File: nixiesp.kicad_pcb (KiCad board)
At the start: 2 copper layers, 152.4 x 53.3 mm, 51 parts, among them J1 Power 9-15V, J2 ESP8266, J3 Nixie PSU low, J4 CONN_01X02, Q1 BS107, Q2 BS107, Q3 BS107, Q4 BS107, U1 74HC595, U10 LM1117-3.3, U11 LM1117-3.3, U2 K155ID1, U3 K155ID1, U4 K155ID1, U5 74HC595, U6 K155ID1, U7 K155ID1, U8 74HC595, U9 K155ID1

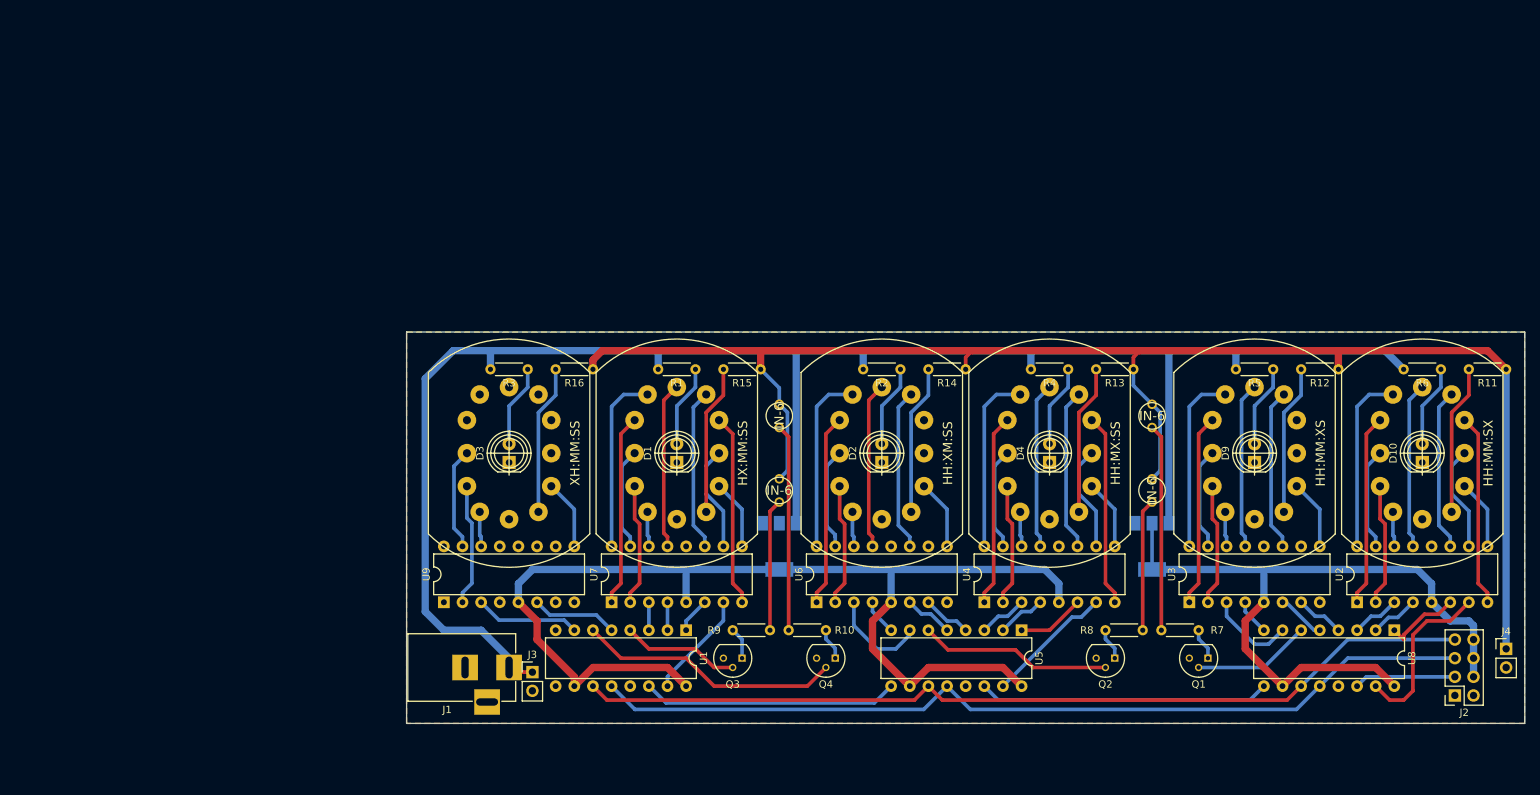
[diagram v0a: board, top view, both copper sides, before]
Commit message: Hopefully final changes
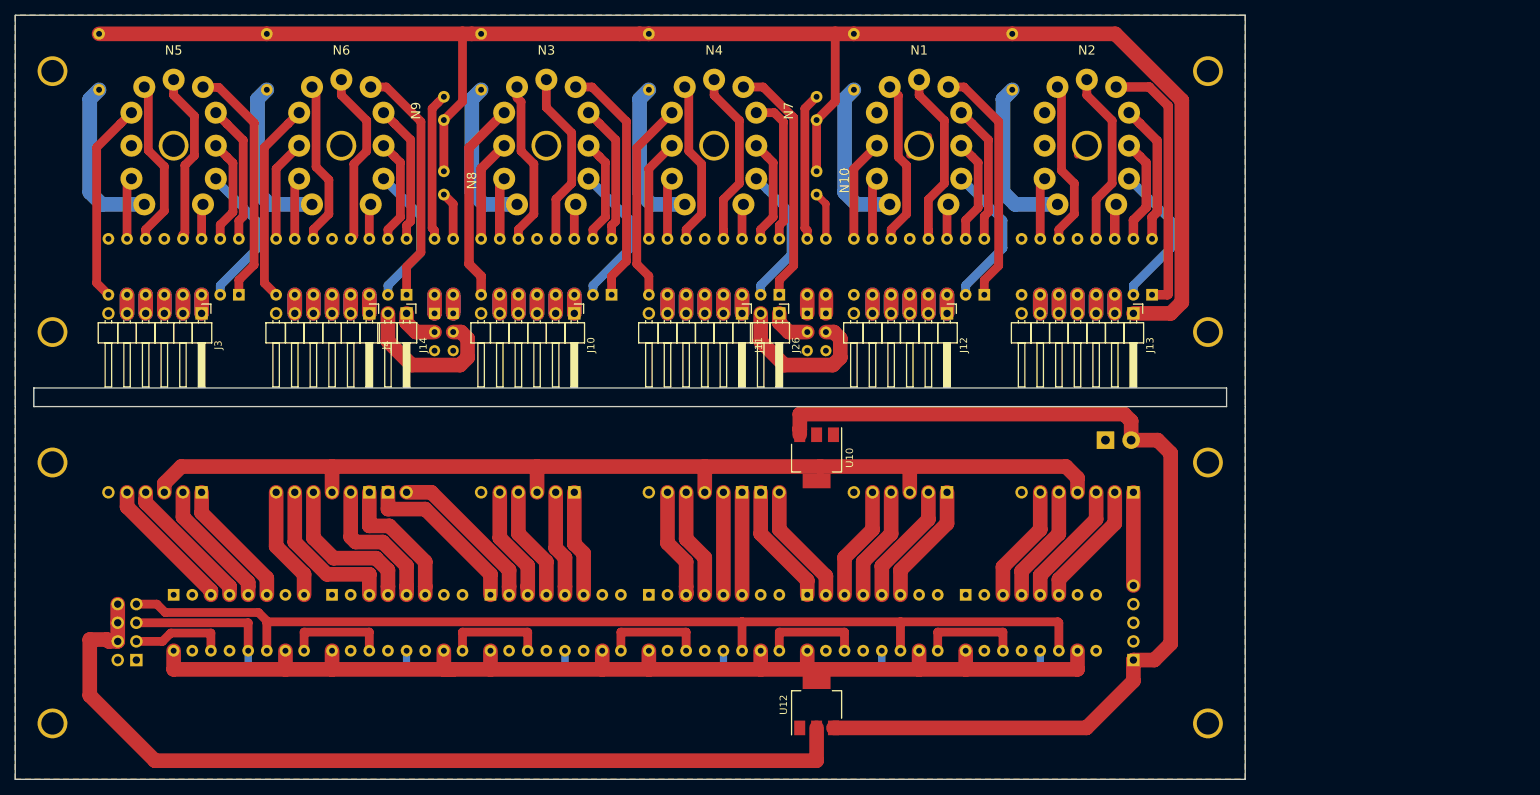
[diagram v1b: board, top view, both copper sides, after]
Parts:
- removed D1, D10, D2, D3, D4, D9: LED, LEDs:LED_D5.0mm
- removed R1, R2, R3, R4, R5, R6: 330, Resistors_THT:R_Axial_DIN0204_L3.6mm_D1.6mm_P5.08mm_Horizontal
- added J10: CONN_01X06, Pin_Headers:Pin_Header_Angled_1x06_Pitch2.54mm, F.Cu at (101.6, 66.0)
- added J11: CONN_01X06, Pin_Headers:Pin_Header_Angled_1x06_Pitch2.54mm, F.Cu at (124.5, 66.0)
- added J12: CONN_01X06, Pin_Headers:Pin_Header_Angled_1x06_Pitch2.54mm, F.Cu at (152.4, 66.0)
- added J13: CONN_01X07, Pin_Headers:Pin_Header_Angled_1x07_Pitch2.54mm, F.Cu at (177.8, 66.0)
- added J14: CONN_01X02, Pin_Headers:Pin_Header_Angled_1x02_Pitch2.54mm, F.Cu at (78.7, 66.0)
- added J15: CONN_01X01, Connectors:1pin, B.Cu at (148.6, 43.2)
- added J16: CONN_01X01, Connectors:1pin, B.Cu at (69.8, 43.2)
- added J17: CONN_01X01, Connectors:1pin, B.Cu at (171.4, 43.2)
- added J18: CONN_01X01, Connectors:1pin, B.Cu at (120.7, 43.2)
- added J19: CONN_01X01, Connectors:1pin, B.Cu at (47.0, 43.2)
- added J20: CONN_01X01, Connectors:1pin, B.Cu at (97.8, 43.2)
- added J21: CONN_01X01, Connectors:1pin, B.Cu at (188.0, 121.9)
- added J22: CONN_01X01, Connectors:1pin, B.Cu at (30.5, 68.6)
- added J23: CONN_01X01, Connectors:1pin, B.Cu at (30.5, 121.9)
- added J24: CONN_01X01, Connectors:1pin, B.Cu at (188.0, 86.4)
- added J25: CONN_01X01, Connectors:1pin, B.Cu at (30.5, 86.4)
- added J26: CONN_01X02, Pin_Headers:Pin_Header_Angled_1x02_Pitch2.54mm, F.Cu at (129.5, 66.0)
- added J27: CONN_01X06, Socket_Strips:Socket_Strip_Straight_1x06_Pitch2.54mm, B.Cu at (50.8, 90.4)
- added J28: CONN_01X06, Socket_Strips:Socket_Strip_Straight_1x06_Pitch2.54mm, B.Cu at (73.7, 90.4)
- added J29: CONN_01X06, Socket_Strips:Socket_Strip_Straight_1x06_Pitch2.54mm, B.Cu at (101.6, 90.4)
- added J30: CONN_01X06, Socket_Strips:Socket_Strip_Straight_1x06_Pitch2.54mm, B.Cu at (124.5, 90.4)
- added J31: CONN_01X07, Socket_Strips:Socket_Strip_Straight_1x07_Pitch2.54mm, B.Cu at (177.8, 90.4)
- added J32: CONN_01X02, Socket_Strips:Socket_Strip_Straight_1x02_Pitch2.54mm, B.Cu at (76.2, 90.4)
- added J33: CONN_01X02, Socket_Strips:Socket_Strip_Straight_1x02_Pitch2.54mm, B.Cu at (127.0, 90.4)
- added J5: CONN_01X06, Socket_Strips:Socket_Strip_Straight_1x06_Pitch2.54mm, B.Cu at (152.4, 90.4)
- added J6: CONN_01X01, Connectors:1pin, B.Cu at (188.0, 68.6)
- added J7: CONN_01X01, Connectors:1pin, B.Cu at (188.0, 33.0)
- added J8: CONN_01X01, Connectors:1pin, B.Cu at (30.5, 33.0)
- added J9: CONN_01X05, Socket_Strips:Socket_Strip_Straight_1x05_Pitch2.54mm, B.Cu at (177.8, 113.3)
- added U12: LM1117-3.3, TO_SOT_Packages_SMD:SOT-223, F.Cu at (134.6, 119.4)
- added U13: 74HC595, Housings_DIP:DIP-16_W7.62mm, B.Cu at (68.6, 104.4)
- added U14: 74HC595, Housings_DIP:DIP-16_W7.62mm, B.Cu at (154.9, 104.4)
- J1: footprint Connectors:BARREL_JACK -> Connectors_Terminal_Blocks:TerminalBlock_Pheonix_PT-3.5mm_2pol; moved to B.Cu
- J2, N1, N10, N2, N3, N4, N5, N6, N7, N8, N9, U1, U2, U3, U4, U5, U6, U7, U8, U9: moved to B.Cu
- J3: value Nixie PSU low -> CONN_01X06; footprint Pin_Headers:Pin_Header_Straight_1x02_Pitch2.54mm -> Pin_Headers:Pin_Header_Angled_1x06_Pitch2.54mm
- J4: value CONN_01X02 -> CONN_01X06; footprint Pin_Headers:Pin_Header_Straight_1x02_Pitch2.54mm -> Pin_Headers:Pin_Header_Angled_1x06_Pitch2.54mm
- Q1, Q2, Q3, Q4: footprint TO_SOT_Packages_THT:TO-92_Molded_Narrow -> TO_SOT_Packages_THT:TO-92_Inline_Wide; moved to B.Cu
- R10, R11, R12, R13, R14, R15, R16, R7, R8, R9: footprint Resistors_THT:R_Axial_DIN0204_L3.6mm_D1.6mm_P5.08mm_Horizontal -> Resistors_THT:R_Axial_DIN0207_L6.3mm_D2.5mm_P7.62mm_Horizontal; moved to B.Cu
- U10: value LM1117-3.3 -> LM1117-5.0; moved to F.Cu
- U11: value LM1117-3.3 -> 74HC595; footprint TO_SOT_Packages_SMD:SOT-223 -> Housings_DIP:DIP-16_W7.62mm
- moved R11 197.1 mm to (36.8, 27.9), turned to 270 degrees
- moved J2 179.8 mm to (41.9, 113.3), turned to 0 degrees
- moved N5 175.3 mm to (47.0, 43.2), turned to 180 degrees
- moved U8 166.4 mm to (47.0, 104.4)
- moved J4 161.5 mm to (73.7, 66.0), turned to 270 degrees
- moved U2 158.1 mm to (55.9, 63.5)
- moved R12 153.0 mm to (59.7, 27.9), turned to 270 degrees
- moved N6 131.3 mm to (69.8, 43.2), turned to 180 degrees
- moved U3 114.6 mm to (78.7, 63.5)
- moved Q1 113.1 mm to (85.1, 66.0), turned to 270 degrees
- moved R7 110.3 mm to (85.1, 55.9), turned to 270 degrees
- moved R8 110.3 mm to (82.5, 55.9), turned to 270 degrees
- moved N9 109.7 mm to (83.8, 38.1), turned to 90 degrees
- moved U9 105.2 mm to (180.3, 63.5)
- moved Q2 103.9 mm to (82.5, 66.0), turned to 270 degrees
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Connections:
- net Net-(J2-Pad3) renamed /data
- J1 pad 1: Net-(J1-Pad1) -> GND
- J1 pad 2: GND -> Net-(J1-Pad2)
- J2 pad 5: Net-(J2-Pad5) -> /latch
- J2 pad 7: Net-(J2-Pad7) -> /clock
- J3 pad 1: Net-(J1-Pad1) -> Net-(J3-Pad1)
- J3 pad 2: GND -> Net-(J3-Pad2)
- J4 pad 2: GND -> Net-(J4-Pad2)
- N10 pad A: Net-(J4-Pad1) -> Net-(J13-Pad1)
- N2 pad 4: (no net) -> Net-(N2-Pad4)
- N2 pad 5: (no net) -> Net-(N2-Pad5)
- N2 pad 6: (no net) -> Net-(N2-Pad6)
- N2 pad 7: (no net) -> Net-(N2-Pad7)
- N2 pad 8: (no net) -> Net-(N2-Pad8)
- N2 pad 9: (no net) -> Net-(N2-Pad9)
- N4 pad 8: (no net) -> Net-(N4-Pad8)
- N4 pad 9: (no net) -> Net-(N4-Pad9)
- N6 pad 8: (no net) -> Net-(N6-Pad8)
- N6 pad 9: (no net) -> Net-(N6-Pad9)
- N7 pad A: Net-(J4-Pad1) -> Net-(J13-Pad1)
- N8 pad A: Net-(J4-Pad1) -> Net-(J13-Pad1)
- N9 pad A: Net-(J4-Pad1) -> Net-(J13-Pad1)
- Q1 pad 2: Net-(Q1-Pad2) -> Net-(J14-Pad2)
- Q2 pad 2: Net-(Q2-Pad2) -> Net-(J14-Pad1)
- Q3 pad 2: Net-(Q3-Pad2) -> Net-(J26-Pad2)
- Q4 pad 2: Net-(Q4-Pad2) -> Net-(J26-Pad1)
- R11 pad 1: Net-(J4-Pad1) -> Net-(J13-Pad1)
- R12 pad 1: Net-(J4-Pad1) -> Net-(J13-Pad1)
- R13 pad 1: Net-(J4-Pad1) -> Net-(J13-Pad1)
- R14 pad 1: Net-(J4-Pad1) -> Net-(J13-Pad1)
- R15 pad 1: Net-(J4-Pad1) -> Net-(J13-Pad1)
- R16 pad 1: Net-(J4-Pad1) -> Net-(J13-Pad1)
- U1 pad 1: Net-(U1-Pad1) -> Net-(J33-Pad1)
- U1 pad 11: Net-(J2-Pad7) -> /clock
- U1 pad 12: Net-(J2-Pad5) -> /latch
- U1 pad 15: Net-(U1-Pad15) -> (no net)
- U1 pad 2: Net-(U1-Pad2) -> Net-(J33-Pad2)
- U1 pad 3: Net-(U1-Pad3) -> Net-(J5-Pad5)
- U1 pad 4: Net-(Q3-Pad2) -> Net-(J5-Pad4)
- U1 pad 5: Net-(U1-Pad5) -> Net-(J5-Pad2)
- U1 pad 6: Net-(Q4-Pad2) -> Net-(J5-Pad1)
- U1 pad 7: Net-(U1-Pad7) -> (no net)
- U1 pad 9: (no net) -> Net-(U1-Pad9)
- U10 pad 3: Net-(J1-Pad1) -> Net-(J1-Pad2)
- U11 pad 1: GND -> (no net)
- U11 pad 2: VCC -> (no net)
- U11 pad 3: Net-(J1-Pad1) -> Net-(J30-Pad5)
- U11 pad 4: VCC -> Net-(J30-Pad4)
- U2 pad 1: Net-(N5-Pad4) -> Net-(N5-Pad5)
- U2 pad 10: Net-(N5-Pad9) -> Net-(N5-Pad0)
- U2 pad 16: Net-(N5-Pad5) -> Net-(N5-Pad4)
- U2 pad 3: Net-(U2-Pad3) -> Net-(J3-Pad1)
- U2 pad 4: Net-(U2-Pad4) -> Net-(J3-Pad2)
- U2 pad 6: Net-(U2-Pad6) -> Net-(J3-Pad4)
- U2 pad 7: Net-(U2-Pad7) -> Net-(J3-Pad5)
- U2 pad 9: Net-(N5-Pad0) -> Net-(N5-Pad9)
- U3 pad 1: Net-(N6-Pad4) -> Net-(N6-Pad5)
- U3 pad 10: (no net) -> Net-(N6-Pad0)
- U3 pad 16: Net-(N6-Pad5) -> Net-(N6-Pad4)
- U3 pad 3: Net-(U3-Pad3) -> Net-(J4-Pad1)
- U3 pad 4: GND -> Net-(J4-Pad2)
- U3 pad 6: Net-(U3-Pad6) -> Net-(J4-Pad4)
- U3 pad 7: Net-(U3-Pad7) -> Net-(J4-Pad5)
- U3 pad 8: (no net) -> Net-(N6-Pad8)
- U3 pad 9: Net-(N6-Pad0) -> Net-(N6-Pad9)
- U4 pad 1: Net-(N3-Pad4) -> Net-(N3-Pad5)
- U4 pad 10: Net-(N3-Pad9) -> Net-(N3-Pad0)
- U4 pad 16: Net-(N3-Pad5) -> Net-(N3-Pad4)
- U4 pad 3: Net-(U4-Pad3) -> Net-(J10-Pad1)
- U4 pad 4: Net-(U4-Pad4) -> Net-(J10-Pad2)
- U4 pad 6: Net-(U4-Pad6) -> Net-(J10-Pad4)
- U4 pad 7: Net-(U4-Pad7) -> Net-(J10-Pad5)
- U4 pad 9: Net-(N3-Pad0) -> Net-(N3-Pad9)
- U5 pad 1: Net-(U4-Pad6) -> Net-(J32-Pad1)
- U5 pad 11: Net-(J2-Pad7) -> /clock
- U5 pad 12: Net-(J2-Pad5) -> /latch
- U5 pad 14: Net-(U5-Pad14) -> Net-(U13-Pad9)
- U5 pad 15: Net-(U4-Pad7) -> (no net)
- U5 pad 2: Net-(U4-Pad4) -> Net-(J32-Pad2)
- U5 pad 3: Net-(U4-Pad3) -> Net-(J29-Pad5)
- U5 pad 4: Net-(U5-Pad4) -> Net-(J29-Pad4)
- U5 pad 5: Net-(U5-Pad5) -> Net-(J29-Pad2)
- U5 pad 6: Net-(Q2-Pad2) -> Net-(J29-Pad1)
- U5 pad 7: Net-(U5-Pad7) -> (no net)
- U5 pad 9: Net-(U1-Pad14) -> Net-(U11-Pad14)
- U6 pad 1: Net-(N4-Pad4) -> Net-(N4-Pad5)
- U6 pad 10: (no net) -> Net-(N4-Pad0)
- U6 pad 16: Net-(N4-Pad5) -> Net-(N4-Pad4)
- U6 pad 3: Net-(U5-Pad7) -> Net-(J11-Pad1)
- U6 pad 4: GND -> Net-(J11-Pad2)
- U6 pad 6: Net-(U5-Pad5) -> Net-(J11-Pad4)
- U6 pad 7: Net-(U5-Pad4) -> Net-(J11-Pad5)
- U6 pad 8: (no net) -> Net-(N4-Pad8)
- U6 pad 9: Net-(N4-Pad0) -> Net-(N4-Pad9)
- U7 pad 1: Net-(N1-Pad4) -> Net-(N1-Pad5)
- U7 pad 10: Net-(N1-Pad9) -> Net-(N1-Pad0)
- U7 pad 16: Net-(N1-Pad5) -> Net-(N1-Pad4)
- U7 pad 3: Net-(U1-Pad3) -> Net-(J12-Pad1)
- U7 pad 4: Net-(U1-Pad2) -> Net-(J12-Pad2)
- U7 pad 6: Net-(U1-Pad1) -> Net-(J12-Pad4)
- U7 pad 7: Net-(U1-Pad15) -> Net-(J12-Pad5)
- U7 pad 9: Net-(N1-Pad0) -> Net-(N1-Pad9)
- U8 pad 1: Net-(U2-Pad6) -> (no net)
- U8 pad 11: Net-(J2-Pad7) -> /clock
- U8 pad 12: Net-(J2-Pad5) -> /latch
- U8 pad 15: Net-(U2-Pad7) -> (no net)
- U8 pad 2: Net-(U2-Pad4) -> (no net)
- U8 pad 3: Net-(U2-Pad3) -> Net-(J27-Pad5)
- U8 pad 4: Net-(U3-Pad7) -> Net-(J27-Pad4)
- U8 pad 5: Net-(U3-Pad6) -> Net-(J27-Pad2)
- U8 pad 6: Net-(Q1-Pad2) -> Net-(J27-Pad1)
- U8 pad 7: Net-(U3-Pad3) -> (no net)
- U8 pad 9: Net-(U5-Pad14) -> Net-(U13-Pad14)
- U9 pad 1: (no net) -> Net-(N2-Pad5)
- U9 pad 10: (no net) -> Net-(N2-Pad0)
- U9 pad 11: (no net) -> Net-(N2-Pad7)
- U9 pad 13: (no net) -> Net-(N2-Pad6)
- U9 pad 16: (no net) -> Net-(N2-Pad4)
- U9 pad 3: Net-(U1-Pad7) -> Net-(J13-Pad2)
- U9 pad 4: GND -> Net-(J13-Pad3)
- U9 pad 6: Net-(U1-Pad5) -> Net-(J13-Pad5)
- U9 pad 7: GND -> Net-(J13-Pad6)
- U9 pad 8: (no net) -> Net-(N2-Pad8)
- U9 pad 9: Net-(N2-Pad0) -> Net-(N2-Pad9)
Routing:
- net Net-(J1-Pad1): track 246.7 -> 0.00 mm
- net Net-(J13-Pad1): track 0.00 -> 225.6 mm
- net Net-(J4-Pad1): track 210.1 -> 5.08 mm
- net VCC: track 249.3 -> 452.8 mm
- net /clock: track 0.00 -> 142.5 mm
- net /latch: track 0.00 -> 142.2 mm
- net Net-(J1-Pad2): track 0.00 -> 135.4 mm
- net Net-(J2-Pad7): track 123.3 -> 0.00 mm
- net Net-(J2-Pad5): track 121.8 -> 0.00 mm
- net Net-(U5-Pad14): track 39.7 -> 0.00 mm
- net Net-(Q4-Pad2): track 36.6 -> 0.00 mm
- net Net-(N2-Pad5): track 0.00 -> 36.0 mm
- net Net-(N4-Pad8): track 0.00 -> 27.5 mm
- net Net-(N6-Pad8): track 0.00 -> 27.4 mm
- net Net-(Q2-Pad2): track 26.2 -> 0.00 mm
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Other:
- board size 152.4 x 53.3 mm -> 167.6 x 104.1 mm
- net class Default: trace_width 0.5 -> 1
- rule trace_min: 0.5 -> 1
